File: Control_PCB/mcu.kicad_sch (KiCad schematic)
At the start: 8 parts, among them U1 STM32G473VET3

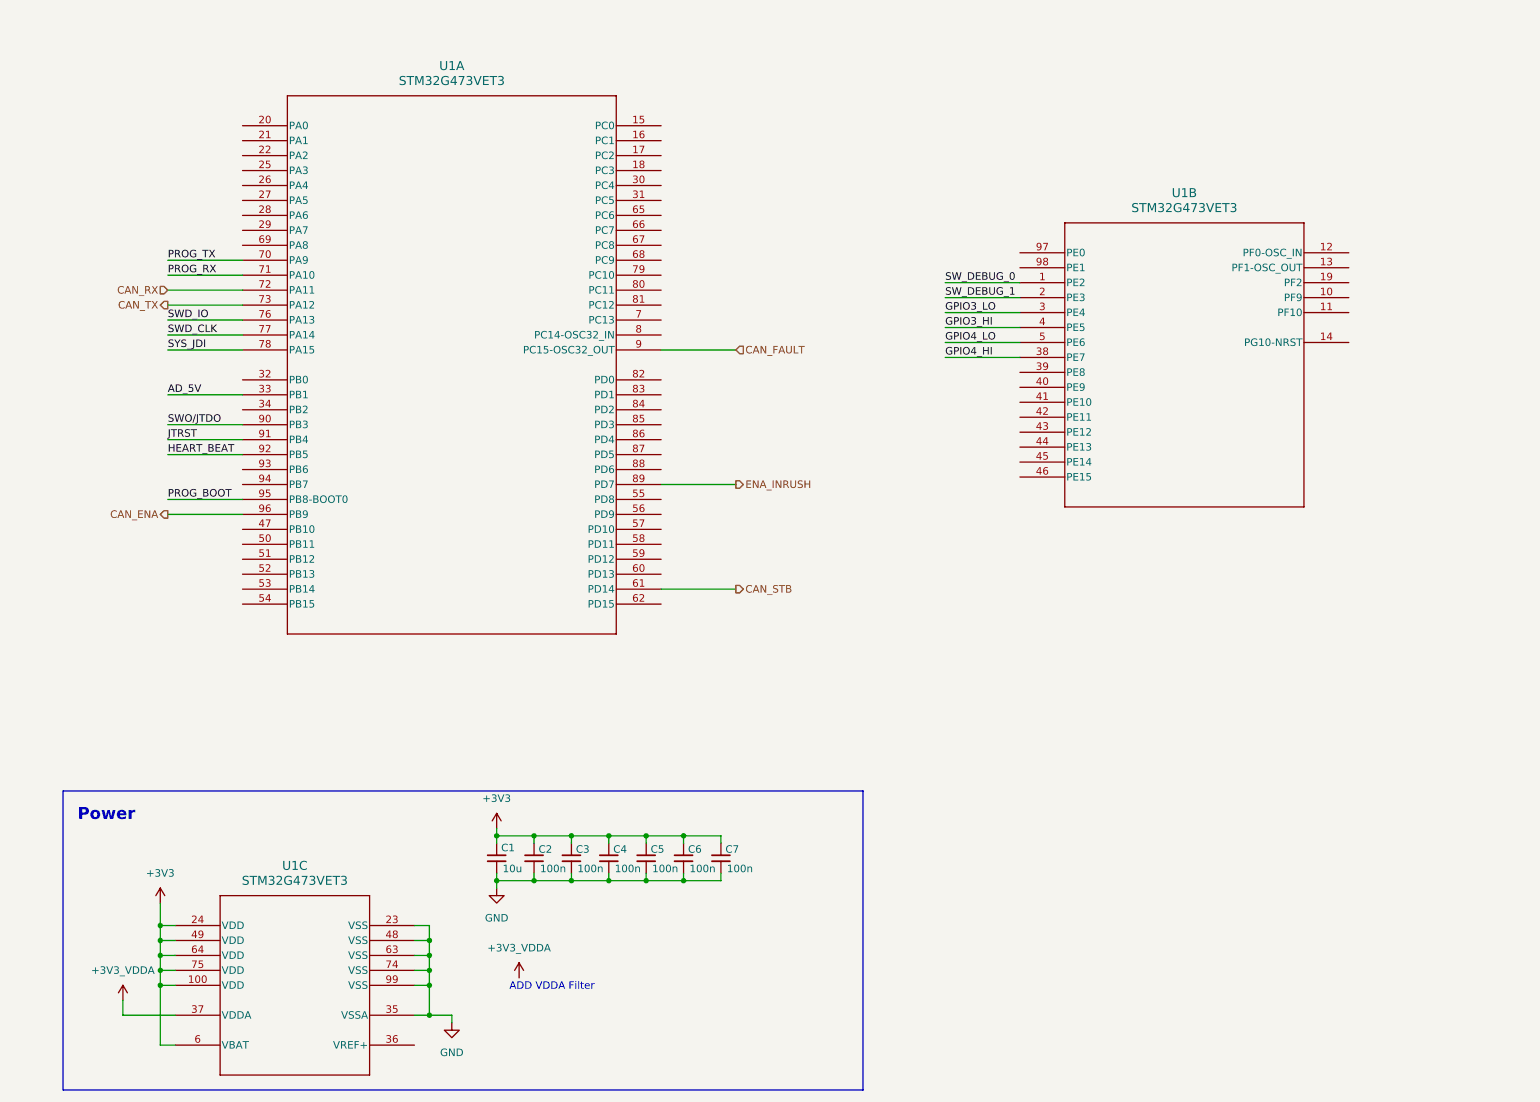
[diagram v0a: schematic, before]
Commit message: 07-20-2026
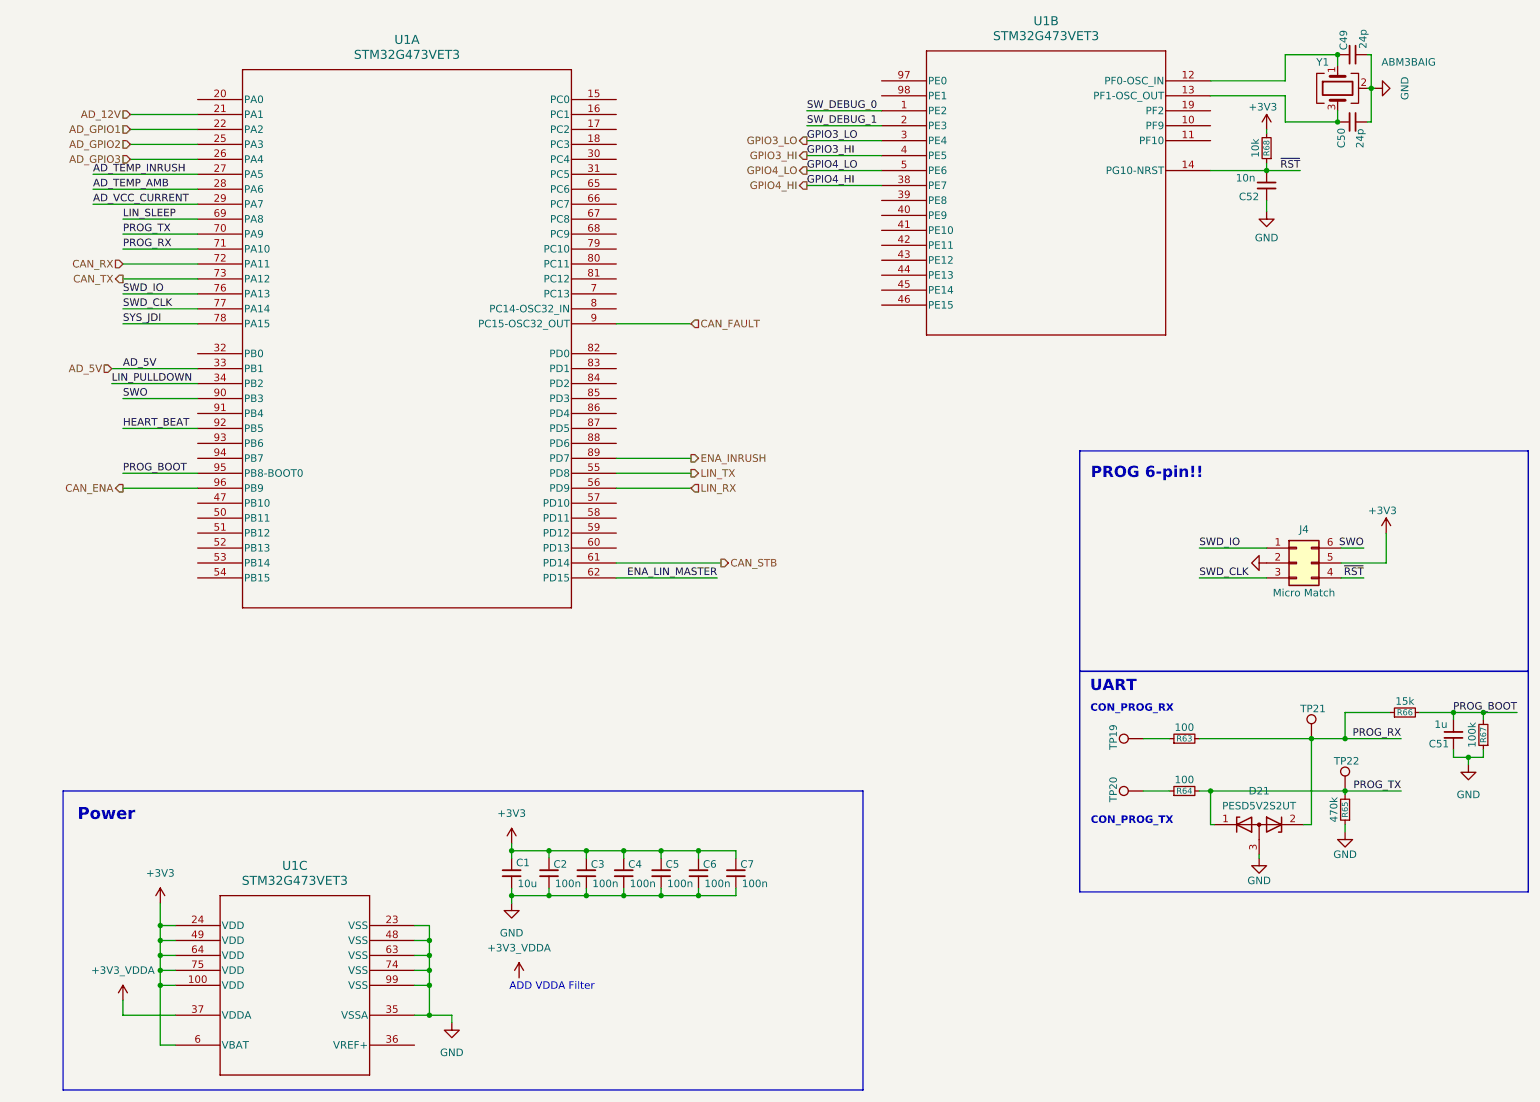
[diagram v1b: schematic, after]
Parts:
- added C49, C50: 24p, Capacitor_SMD:C_0603_1608Metric, symbol Device:C_Small
- added C51: 1u, Capacitor_SMD:C_0603_1608Metric, symbol Device:C_Small
- added C52: 10n, Capacitor_SMD:C_0603_1608Metric, symbol Device:C_Small
- added D21: PESD5V2S2UT, Package_TO_SOT_SMD:SOT-23, symbol Device:D_Zener_Dual_CommonAnode_KKA
- added J4: Micro Match, Connector_Molex:Molex_Mini-Fit_Jr_5569-06A2_2x03_P4.20mm_Horizontal, symbol Connector_Generic:Conn_02x03_Counter_Clockwise
- added R63, R64: 100, symbol Device:R_Small
- added R65: 470k, symbol Device:R_Small
- added R66: 15k, symbol Device:R_Small
- added R67: 100k, Resistor_SMD:R_0603_1608Metric, symbol Device:R_Small
- added R68: 10k, symbol Device:R_Small
- added TP19, TP20, TP21, TP22: TestPoint, TestPoint:TestPoint_Pad_D1.5mm, symbol Connector:TestPoint
- added Y1: ABM3BAIG, Crystal:Crystal_SMD_5032-4Pin_5.0x3.2mm, symbol Device:Crystal_GND24
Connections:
- net +3V3: now also J4.5 (Pin_5), R68.2
- net GND: now also C49.2, C50.2, C51.1, C52.1, D21.3 (A), J4.2 (Pin_2), R65.1, R67.1, Y1.2 (G), Y1.4 (G)
- net PROG_BOOT: now also C51.2, R66.2, R67.2
- net PROG_RX: now also D21.2 (K), R63.2, R66.1, TP21.1
- net PROG_TX: now also D21.1 (K), R64.2, R65.2, TP22.1
- net SWD_CLK: now also J4.3 (Pin_3)
- net SWD_IO: now also J4.1 (Pin_1)
- net AD_12V: now reaches U1.21 (PA1)
- net AD_GPIO1: now reaches U1.22 (PA2)
- net AD_GPIO2: now reaches U1.25 (PA3)
- net AD_GPIO3: now reaches U1.26 (PA4)
- net AD_TEMP_INRUSH: now reaches U1.27 (PA5)
- net AD_TEMP_AMB: now reaches U1.28 (PA6)
- net AD_VCC_CURRENT: now reaches U1.29 (PA7)
- net LIN_PULLDOWN: now reaches U1.34 (PB2)
- net LIN_TX: now reaches U1.55 (PD8)
- net LIN_RX: now reaches U1.56 (PD9)
- net ENA_LIN_MASTER: now reaches U1.62 (PD15)
- net LIN_SLEEP: now reaches U1.69 (PA8)
- net at U1.12 (PF0-OSC_IN): now also C49.1, Y1.1
- net at U1.13 (PF1-OSC_OUT): now also C50.1, Y1.3
- net ~{RST}: now reaches U1.14 (PG10-NRST)
- net ~{RST}: now also C52.2, J4.4 (Pin_4), R68.1
- net JTRST: no longer names the net of U1.91 (PB4)
- net SWO/JTDO renamed SWO
- net SWO: now also J4.6 (Pin_6)
- new net: R64.1, TP20.1
- new net: R63.1, TP19.1
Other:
- note added: "CON_PROG_RX"
- note added: "CON_PROG_TX"
- note added: "PROG 6-pin!!"
- note added: "UART"
- moved on the sheet: C1, C2, C3, C4, C5, C6, C7, U1A, U1B

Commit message: 10-10-2026
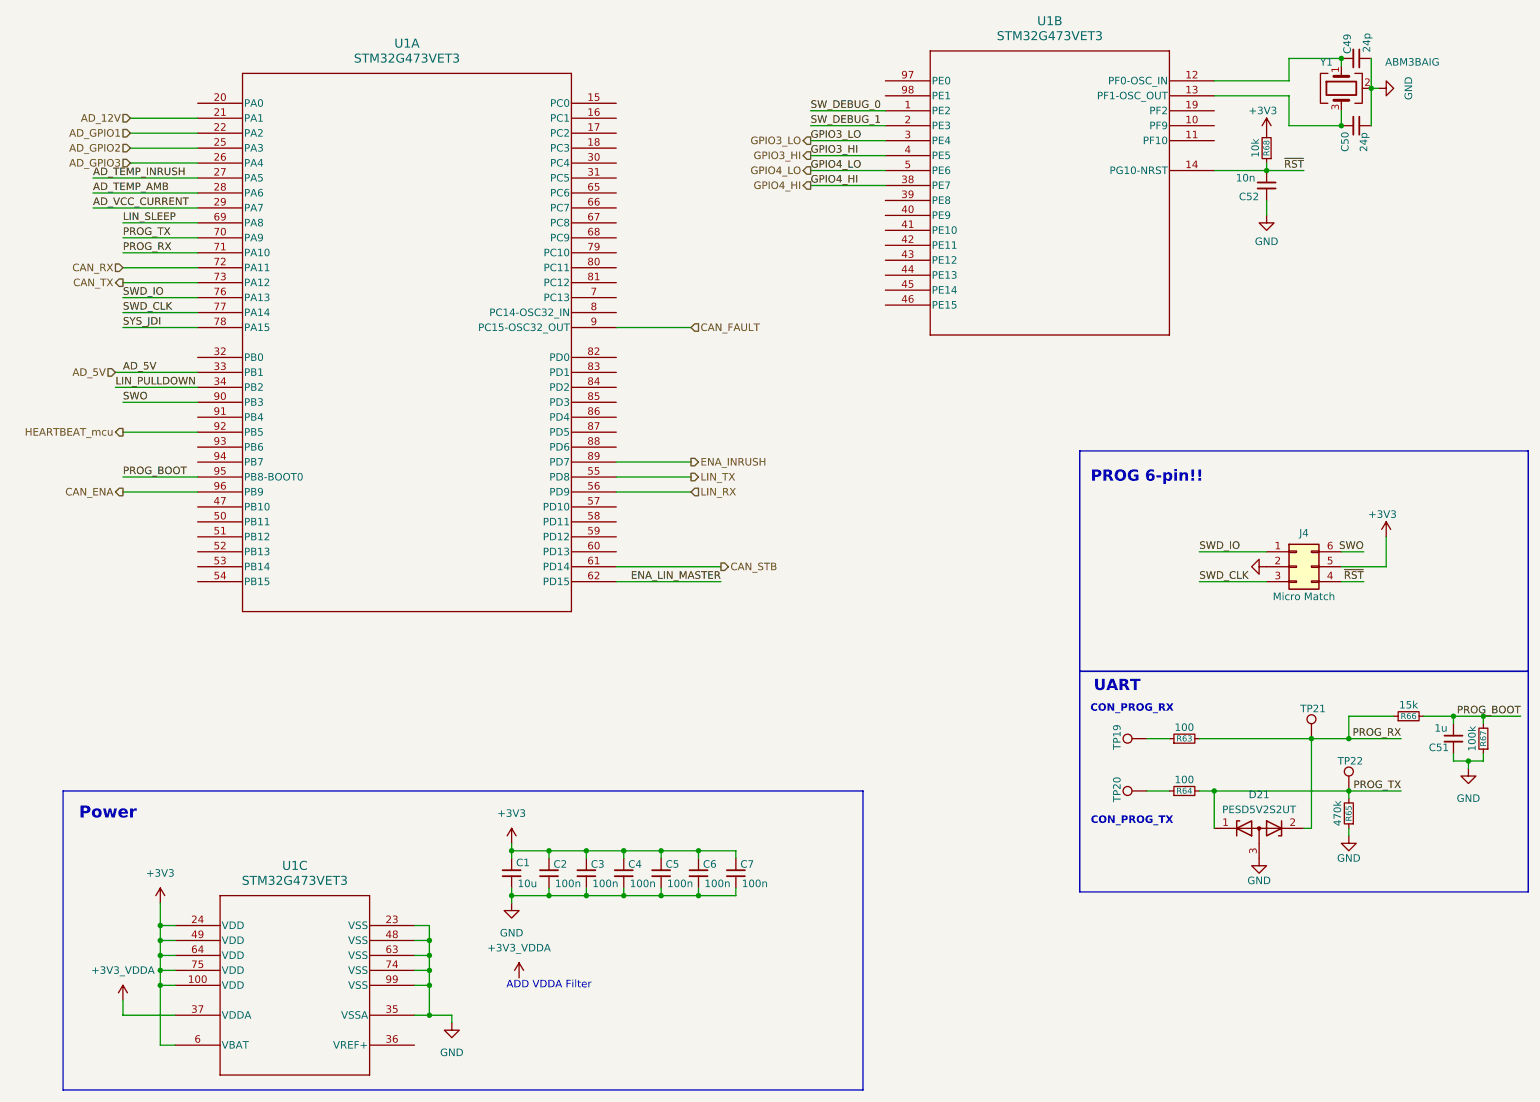
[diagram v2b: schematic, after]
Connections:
- net HEART_BEAT renamed HEARTBEAT_mcu
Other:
- moved on the sheet: C49, C50, C51, D21, J4, R65, R66, R67, TP19, TP20, TP22, U1A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

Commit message: Before removing stuffs
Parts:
- J4: footprint Connector_Molex:Molex_Mini-Fit_Jr_5569-06A2_2x03_P4.20mm_Horizontal -> Control_PCB:CONN6_7-188275-6_TEC
- R63, R64, R65, R66, R68: footprint (none) -> Resistor_SMD:R_0603_1608Metric
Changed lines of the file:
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@@
 			)
 		)
-		(property "Footprint" "Connector_Molex:Molex_Mini-Fit_Jr_5569-06A2_2x03_P4.20mm_Horizontal"
+		(property "Footprint" "Control_PCB:CONN6_7-188275-6_TEC"
 			(at 232.41 105.41 0)
 			(hide yes)
@@
 			)
 		)
-		(property "Footprint" ""
+		(property "Footprint" "Resistor_SMD:R_0603_1608Metric"
 			(at 213.36 143.51 0)
 			(hide yes)
@@
 			)
 		)
-		(property "Footprint" ""
+		(property "Footprint" "Resistor_SMD:R_0603_1608Metric"
 			(at 251.46 130.81 0)
 			(hide yes)
@@
 			)
 		)
-		(property "Footprint" ""
+		(property "Footprint" "Resistor_SMD:R_0603_1608Metric"
 			(at 227.33 34.29 0)
 			(hide yes)
@@
 			)
 		)
-		(property "Footprint" ""
+		(property "Footprint" "Resistor_SMD:R_0603_1608Metric"
 			(at 241.3 147.32 0)
 			(hide yes)
@@
 			)
 		)
-		(property "Footprint" ""
+		(property "Footprint" "Resistor_SMD:R_0603_1608Metric"
 			(at 213.36 134.62 0)
 			(hide yes)
